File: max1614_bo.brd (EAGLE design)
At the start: 14 x 10.2 mm, 4 parts, among them IC1 MAX1614

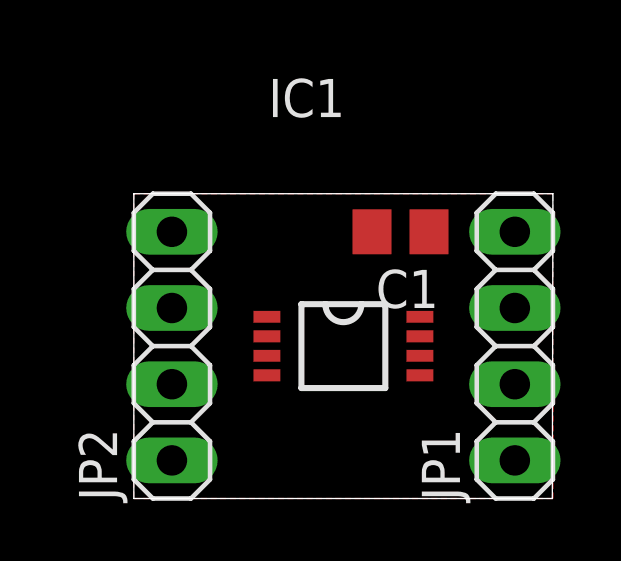
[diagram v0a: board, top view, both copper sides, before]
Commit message: routed
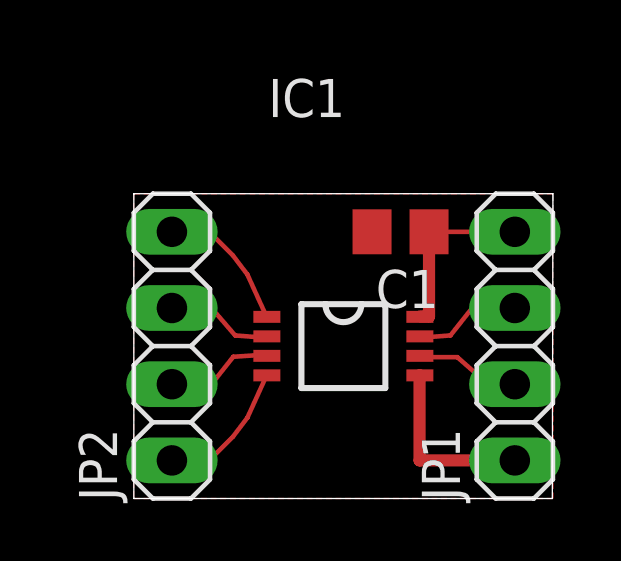
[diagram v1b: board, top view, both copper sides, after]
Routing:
- net BAT: track 0.00 -> 6.28 mm
- net GND: track 0.00 -> 6.02 mm
- net LBI: track 0.00 -> 4.71 mm
- net -ON: track 0.00 -> 4.71 mm
- net SRC: track 0.00 -> 3.62 mm
- net -LBO: track 0.00 -> 3.62 mm
- net -OFF: track 0.00 -> 3.59 mm
- net GATE: track 0.00 -> 3.53 mm
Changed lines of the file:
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@@
 <setting verticaltext="up"/>
 </settings>
-<grid distance="50" unitdist="mil" unit="mil" style="lines" multiple="1" display="yes" altdistance="0.025" altunitdist="inch" altunit="mil"/>
+<grid distance="2.5" unitdist="mil" unit="mil" style="lines" multiple="1" display="yes" altdistance="0.025" altunitdist="inch" altunit="mil"/>
 <layers>
 <layer number="1" name="Top" color="4" fill="1" visible="yes" active="yes"/>
@@
 <autorouter>
 <pass name="Default">
-<param name="RoutingGrid" value="50mil"/>
+<param name="RoutingGrid" value="1mil"/>
 <param name="tpViaShape" value="round"/>
-<param name="PrefDir.1" value="|"/>
+<param name="PrefDir.1" value="-"/>
 <param name="PrefDir.2" value="0"/>
 <param name="PrefDir.3" value="0"/>
@@
 <param name="PrefDir.14" value="0"/>
 <param name="PrefDir.15" value="0"/>
-<param name="PrefDir.16" value="-"/>
+<param name="PrefDir.16" value="0"/>
 <param name="cfVia" value="8"/>
 <param name="cfNonPref" value="5"/>
@@
 <contactref element="JP2" pad="4"/>
 <contactref element="IC1" pad="1"/>
-<wire x1="4.435" y1="6.055" x2="1.27" y2="8.89" width="0" layer="19" extent="1-1"/>
+<wire x1="3.7846" y1="7.4676" x2="4.4196" y2="6.0706" width="0.1524" layer="1"/>
+<wire x1="3.302" y1="8.1026" x2="3.7846" y2="7.4676" width="0.1524" layer="1"/>
+<wire x1="2.5146" y1="8.89" x2="3.302" y2="8.1026" width="0.1524" layer="1"/>
+<wire x1="1.27" y1="8.89" x2="2.5146" y2="8.89" width="0.1524" layer="1"/>
+<wire x1="4.4196" y1="6.0706" x2="4.435" y2="6.055" width="0.1524" layer="1"/>
 </signal>
 <signal name="-OFF">
 <contactref element="JP2" pad="3"/>
 <contactref element="IC1" pad="2"/>
-<wire x1="1.27" y1="6.35" x2="4.435" y2="5.405" width="0" layer="19" extent="1-1"/>
+<wire x1="4.2037" y1="5.3721" x2="4.4196" y2="5.4102" width="0.1524" layer="1"/>
+<wire x1="3.3782" y1="5.4356" x2="4.2037" y2="5.3721" width="0.1524" layer="1"/>
+<wire x1="2.5908" y1="6.35" x2="3.3782" y2="5.4356" width="0.1524" layer="1"/>
+<wire x1="1.27" y1="6.35" x2="2.5908" y2="6.35" width="0.1524" layer="1"/>
+<wire x1="4.4196" y1="5.4102" x2="4.435" y2="5.405" width="0.1524" layer="1"/>
 </signal>
 <signal name="-LBO">
 <contactref element="JP2" pad="2"/>
 <contactref element="IC1" pad="3"/>
-<wire x1="1.27" y1="3.81" x2="4.435" y2="4.755" width="0" layer="19" extent="1-1"/>
+<wire x1="4.2672" y1="4.7879" x2="4.4196" y2="4.7498" width="0.1524" layer="1"/>
+<wire x1="3.3147" y1="4.7244" x2="4.2672" y2="4.7879" width="0.1524" layer="1"/>
+<wire x1="2.5908" y1="3.81" x2="3.3147" y2="4.7244" width="0.1524" layer="1"/>
+<wire x1="1.27" y1="3.81" x2="2.5908" y2="3.81" width="0.1524" layer="1"/>
+<wire x1="4.4196" y1="4.7498" x2="4.435" y2="4.755" width="0.1524" layer="1"/>
 </signal>
 <signal name="LBI">
 <contactref element="JP2" pad="1"/>
 <contactref element="IC1" pad="4"/>
-<wire x1="1.27" y1="1.27" x2="4.435" y2="4.105" width="0" layer="19" extent="1-1"/>
+<wire x1="3.7846" y1="2.6924" x2="4.4196" y2="4.0894" width="0.1524" layer="1"/>
+<wire x1="3.302" y1="2.0574" x2="3.7846" y2="2.6924" width="0.1524" layer="1"/>
+<wire x1="2.5146" y1="1.27" x2="3.302" y2="2.0574" width="0.1524" layer="1"/>
+<wire x1="1.27" y1="1.27" x2="2.5146" y2="1.27" width="0.1524" layer="1"/>
+<wire x1="4.4196" y1="4.0894" x2="4.435" y2="4.105" width="0.1524" layer="1"/>
 </signal>
 <signal name="BAT">
@@
 <contactref element="JP1" pad="4"/>
 <contactref element="C1" pad="1"/>
-<wire x1="9.84" y1="8.89" x2="12.7" y2="8.89" width="0" layer="19" extent="1-1"/>
-<wire x1="9.535" y1="6.055" x2="9.84" y2="8.89" width="0" layer="19" extent="1-1"/>
+<wire x1="9.8298" y1="8.89" x2="9.5504" y2="8.89" width="0.1524" layer="1"/>
+<wire x1="9.5504" y1="6.0706" x2="9.535" y2="6.055" width="0.1524" layer="1"/>
+<wire x1="9.8298" y1="8.89" x2="9.84" y2="8.89" width="0.1524" layer="1"/>
+<wire x1="12.7" y1="8.89" x2="9.906" y2="8.89" width="0.1524" layer="1"/>
+<wire x1="9.906" y1="8.89" x2="9.84" y2="8.89" width="0.1524" layer="1"/>
+<wire x1="9.5504" y1="6.0706" x2="9.84" y2="6.0706" width="0.4064" layer="1"/>
+<wire x1="9.84" y1="6.0706" x2="9.84" y2="8.89" width="0.4064" layer="1"/>
 </signal>
 <signal name="GATE">
 <contactref element="IC1" pad="6"/>
 <contactref element="JP1" pad="2"/>
-<wire x1="9.535" y1="4.755" x2="12.7" y2="3.81" width="0" layer="19" extent="1-1"/>
+<wire x1="9.6774" y1="4.7117" x2="9.5504" y2="4.7752" width="0.1524" layer="1"/>
+<wire x1="10.7823" y1="4.7117" x2="9.6774" y2="4.7117" width="0.1524" layer="1"/>
+<wire x1="11.811" y1="3.81" x2="10.7823" y2="4.7117" width="0.1524" layer="1"/>
+<wire x1="12.7" y1="3.81" x2="11.811" y2="3.81" width="0.1524" layer="1"/>
+<wire x1="9.5504" y1="4.7752" x2="9.535" y2="4.755" width="0.1524" layer="1"/>
 </signal>
 <signal name="SRC">
 <contactref element="IC1" pad="7"/>
 <contactref element="JP1" pad="3"/>
-<wire x1="9.535" y1="5.405" x2="12.7" y2="6.35" width="0" layer="19" extent="1-1"/>
+<wire x1="9.7028" y1="5.3721" x2="9.5504" y2="5.4102" width="0.1524" layer="1"/>
+<wire x1="10.5537" y1="5.4356" x2="9.7028" y2="5.3721" width="0.1524" layer="1"/>
+<wire x1="11.2776" y1="6.35" x2="10.5537" y2="5.4356" width="0.1524" layer="1"/>
+<wire x1="12.7" y1="6.35" x2="11.2776" y2="6.35" width="0.1524" layer="1"/>
+<wire x1="9.5504" y1="5.4102" x2="9.535" y2="5.405" width="0.1524" layer="1"/>
 </signal>
 <signal name="GND">
-<polygon width="0.4064" layer="1" isolate="0.254">
+<polygon width="0.4064" layer="1" isolate="0.8128">
 <vertex x="0" y="10.16"/>
 <vertex x="0" y="0"/>
@@
 <contactref element="JP1" pad="1"/>
 <contactref element="C1" pad="2"/>
+<wire x1="9.535" y1="4.105" x2="9.525" y2="4.105" width="0.4064" layer="1"/>
+<wire x1="9.525" y1="4.105" x2="9.525" y2="1.27" width="0.4064" layer="1"/>
+<wire x1="9.525" y1="1.27" x2="12.7" y2="1.27" width="0.4064" layer="1"/>
 </signal>
 </signals>
